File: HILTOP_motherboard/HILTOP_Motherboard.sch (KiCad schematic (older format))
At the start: 202 parts, among them J1 BACKPLANE_PWR, J10 HDMI, J11 DISP_PWR, J12 DISPLAY_PORT, J14 VADJ_B, J15 VADJ_A, J16 SOFT_START_PWR, J17 PWR_LED, J18 USB_B, J19 Micro_SD_Card, J2 ATX_MOLEX_02X12, J20 CAMERA_PORT, J21 EXT_FAN, J22 BACKPLANE_LV_PWR, J23 EXT_FAN, J26 IO_EXP, J3 SATA, J4 USB_A_DOUBLE, J5 USB FRONT PANEL, J6 CAN, J7 RS485, J8 EXT_TEMP_MON, J9 RJ45-TRANS_SI-61001-F, U1 LM337BD2TG, U25 STM6719SFWB6F, U39 MCP23017

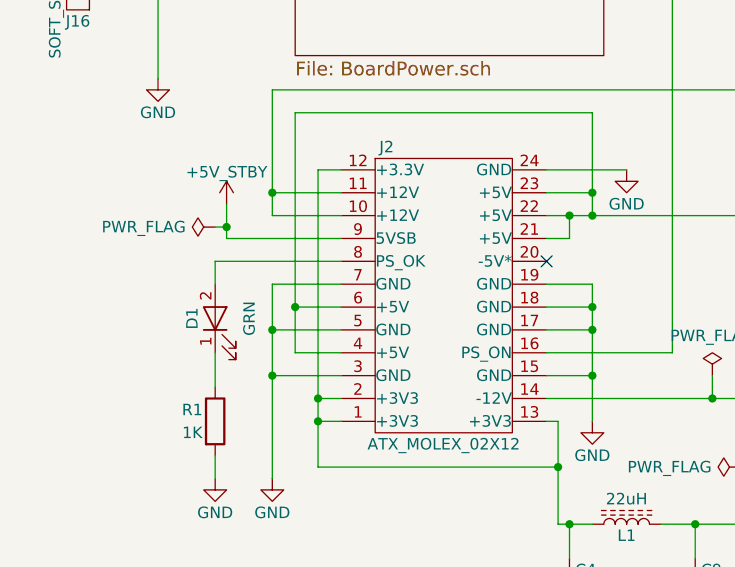
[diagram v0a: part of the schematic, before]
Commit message: nearly there, drc errors all resolved!
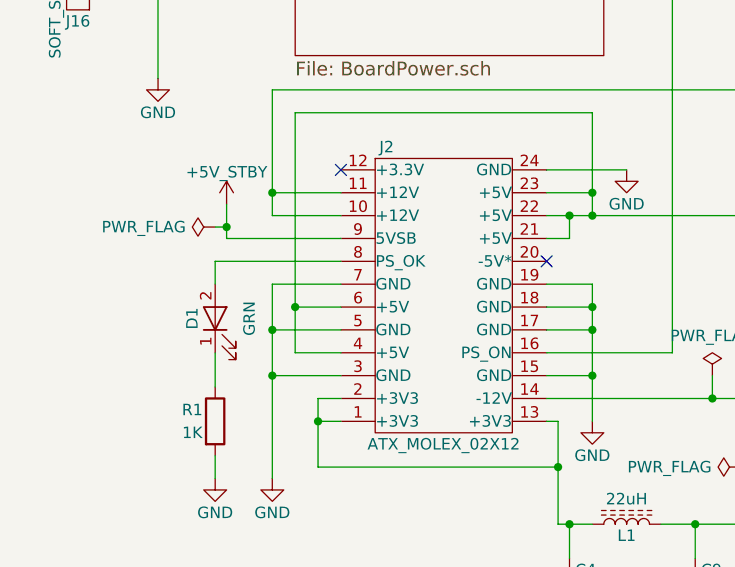
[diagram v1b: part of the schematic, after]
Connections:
- net at C4.1, J2.1 (+3V3), J2.13 (+3V3)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: no longer J2.12 (+3.3V)
- no-connect marks 14 -> 15
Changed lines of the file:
@@
 Wire Wire Line
 	21700 1900 21700 2050
-Connection ~ 2000 14600
-Wire Wire Line
-	2100 13600 2000 13600
 Wire Wire Line
 	3350 13600 3000 13600
@@
 	2000 14700 2100 14700
 Wire Wire Line
-	2000 13600 2000 14600
-Wire Wire Line
 	2000 14900 3050 14900
 Connection ~ 3200 14200
@@
 Wire Wire Line
 	1600 13850 1600 13900
+NoConn ~ 2100 13600
 $EndSCHEMATC
